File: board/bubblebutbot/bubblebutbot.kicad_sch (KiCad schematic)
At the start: 55 parts, among them J1 JST XH, J10 JST XH, J11 JST XH, J13 JST XH, J2 USB_C_Receptacle, J3 Conn_01x03_Socket, J4 Conn_01x03_Socket, J5 Conn_01x03_Socket, J6 Conn_01x03_Socket, J7 Conn_01x03_Socket, J8 Conn_01x03_Socket, J9 JST XH, Q1 FDN336P, SW1 SW_Push, SW2 SW_Push, U1 DRV8833PWP, U2 ESP32-S3-WROOM-1, U3 AP2112K-3.3, U4 LIS3DH

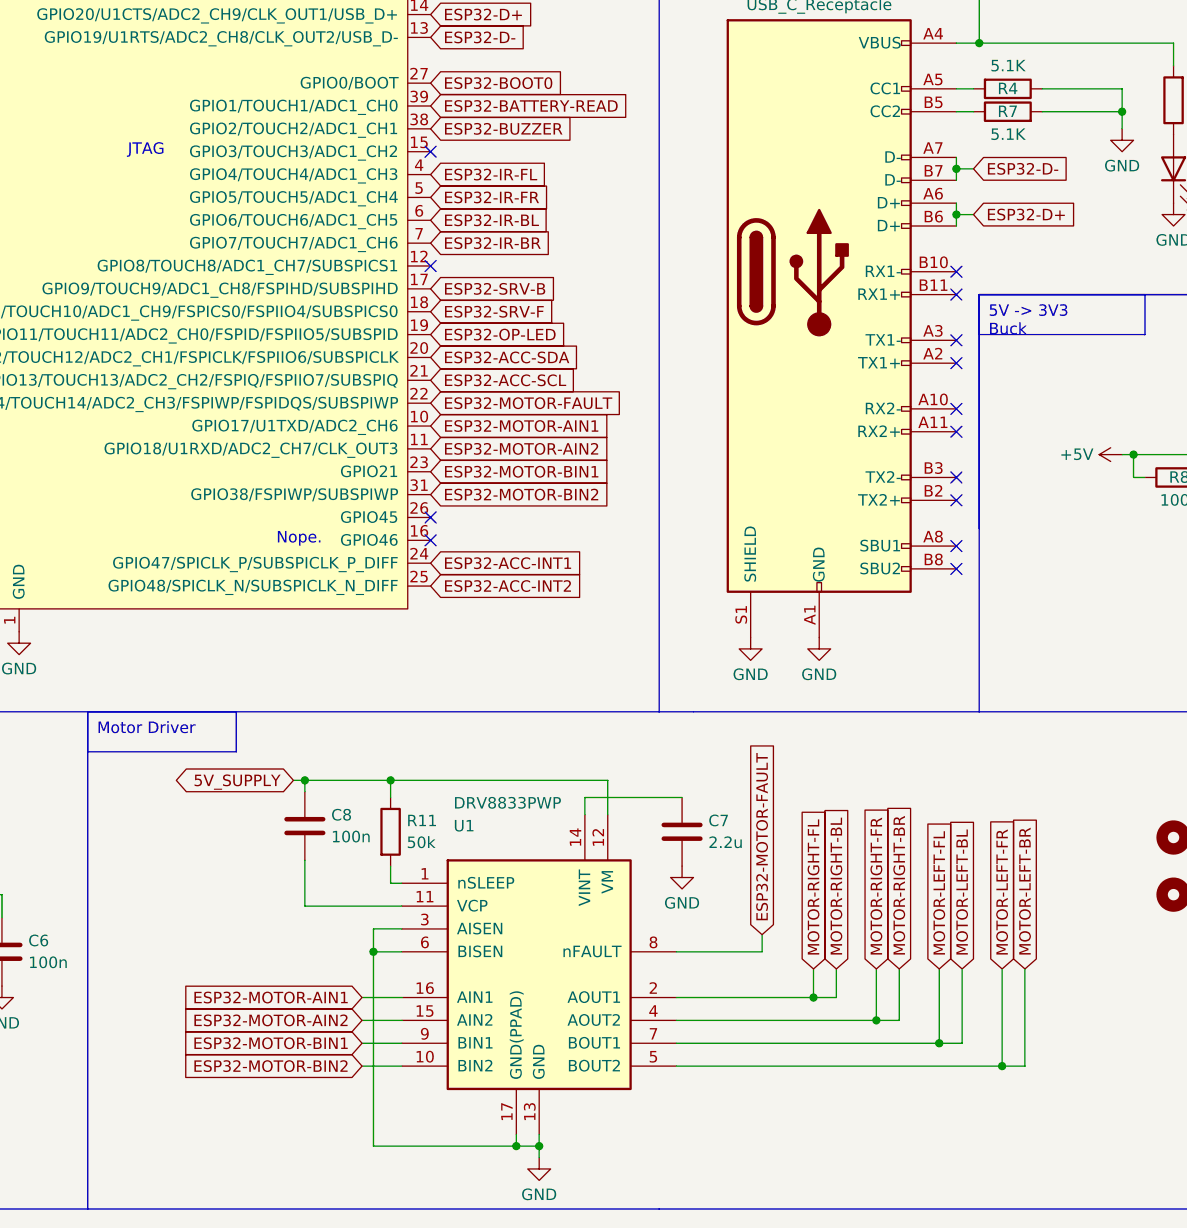
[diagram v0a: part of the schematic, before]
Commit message: pcb done!
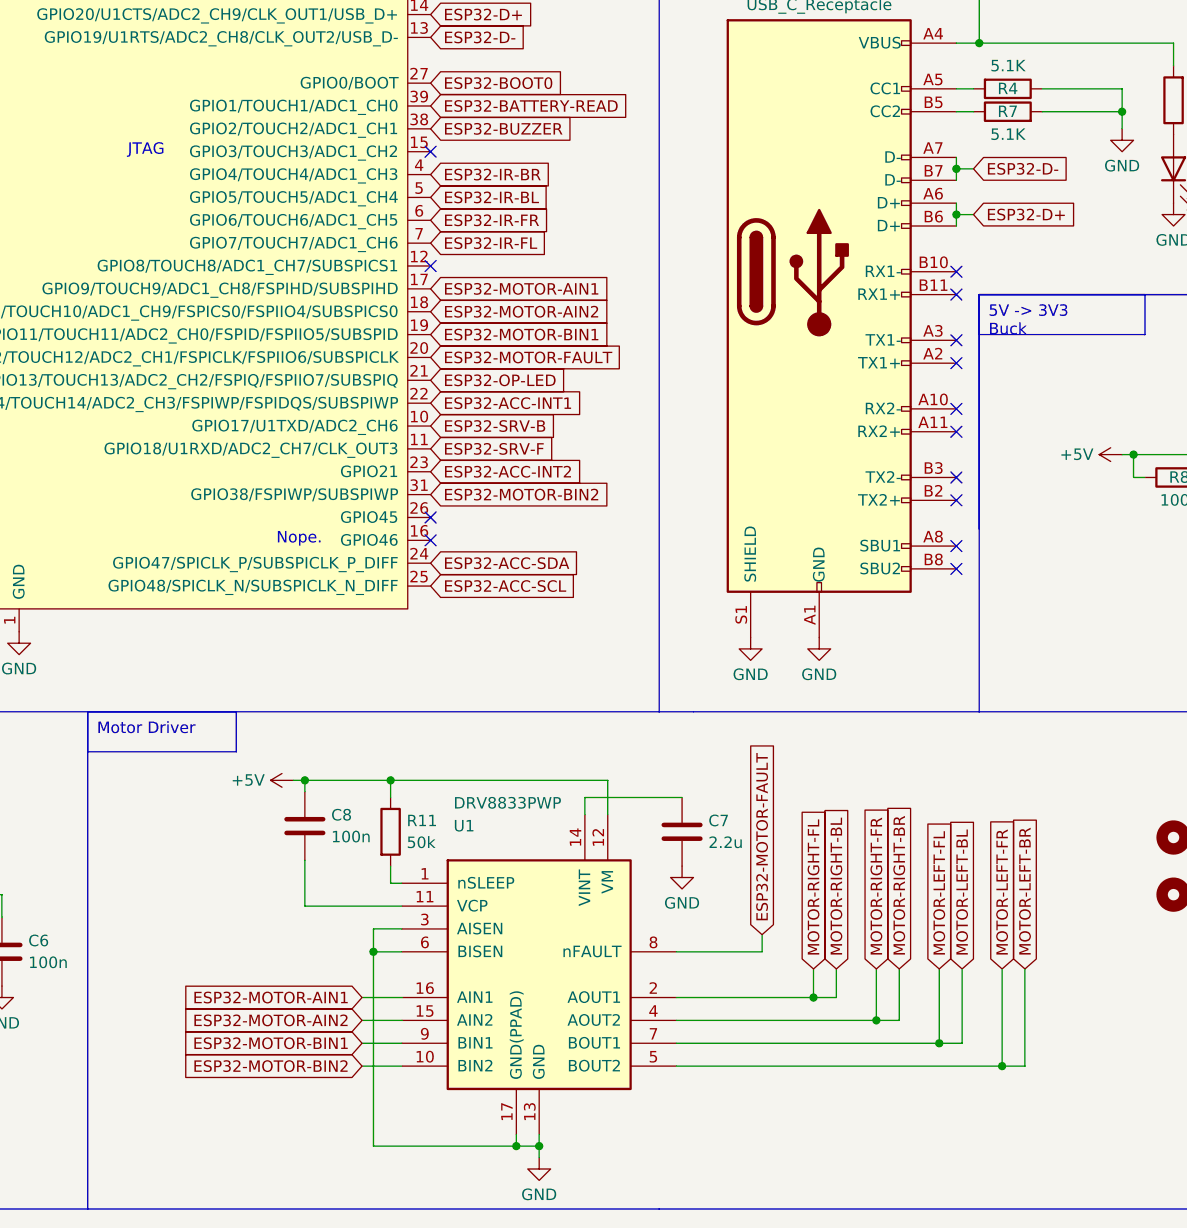
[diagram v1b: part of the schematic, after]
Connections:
- net 5V_SUPPLY is gone; now on net +5V: C8.2, R11.1, U1.12 (VM)
- net ESP32-ACC-INT1: now also U2.22 (GPIO14/TOUCH14/ADC2_CH3/FSPIWP/FSPIDQS/SUBSPIWP); no longer U2.24 (GPIO47/SPICLK_P/SUBSPICLK_P_DIFF)
- net ESP32-ACC-INT2: now also U2.23 (GPIO21); no longer U2.25 (GPIO48/SPICLK_N/SUBSPICLK_N_DIFF)
- net ESP32-ACC-SCL: now also U2.25 (GPIO48/SPICLK_N/SUBSPICLK_N_DIFF); no longer U2.21 (GPIO13/TOUCH13/ADC2_CH2/FSPIQ/FSPIIO7/SUBSPIQ)
- net ESP32-ACC-SDA: now also U2.24 (GPIO47/SPICLK_P/SUBSPICLK_P_DIFF); no longer U2.20 (GPIO12/TOUCH12/ADC2_CH1/FSPICLK/FSPIIO6/SUBSPICLK)
- net ESP32-IR-BL: now also U2.5 (GPIO5/TOUCH5/ADC1_CH4); no longer U2.6 (GPIO6/TOUCH6/ADC1_CH5)
- net ESP32-IR-BR: now also U2.4 (GPIO4/TOUCH4/ADC1_CH3); no longer U2.7 (GPIO7/TOUCH7/ADC1_CH6)
- net ESP32-IR-FL: now also U2.7 (GPIO7/TOUCH7/ADC1_CH6); no longer U2.4 (GPIO4/TOUCH4/ADC1_CH3)
- net ESP32-IR-FR: now also U2.6 (GPIO6/TOUCH6/ADC1_CH5); no longer U2.5 (GPIO5/TOUCH5/ADC1_CH4)
- net ESP32-MOTOR-AIN1: now also U2.17 (GPIO9/TOUCH9/ADC1_CH8/FSPIHD/SUBSPIHD); no longer U2.10 (GPIO17/U1TXD/ADC2_CH6)
- net ESP32-MOTOR-AIN2: now also U2.18 (GPIO10/TOUCH10/ADC1_CH9/FSPICS0/FSPIIO4/SUBSPICS0); no longer U2.11 (GPIO18/U1RXD/ADC2_CH7/CLK_OUT3)
- net ESP32-MOTOR-BIN1: now also U2.19 (GPIO11/TOUCH11/ADC2_CH0/FSPID/FSPIIO5/SUBSPID); no longer U2.23 (GPIO21)
- net ESP32-MOTOR-FAULT: now also U2.20 (GPIO12/TOUCH12/ADC2_CH1/FSPICLK/FSPIIO6/SUBSPICLK); no longer U2.22 (GPIO14/TOUCH14/ADC2_CH3/FSPIWP/FSPIDQS/SUBSPIWP)
- net ESP32-OP-LED: now also U2.21 (GPIO13/TOUCH13/ADC2_CH2/FSPIQ/FSPIIO7/SUBSPIQ); no longer U2.19 (GPIO11/TOUCH11/ADC2_CH0/FSPID/FSPIIO5/SUBSPID)
- net ESP32-SRV-B: now also U2.10 (GPIO17/U1TXD/ADC2_CH6); no longer U2.17 (GPIO9/TOUCH9/ADC1_CH8/FSPIHD/SUBSPIHD)
- net ESP32-SRV-F: now also U2.11 (GPIO18/U1RXD/ADC2_CH7/CLK_OUT3); no longer U2.18 (GPIO10/TOUCH10/ADC1_CH9/FSPICS0/FSPIIO4/SUBSPICS0)
